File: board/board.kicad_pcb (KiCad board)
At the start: 2 copper layers, 21 x 13 mm, 1 part

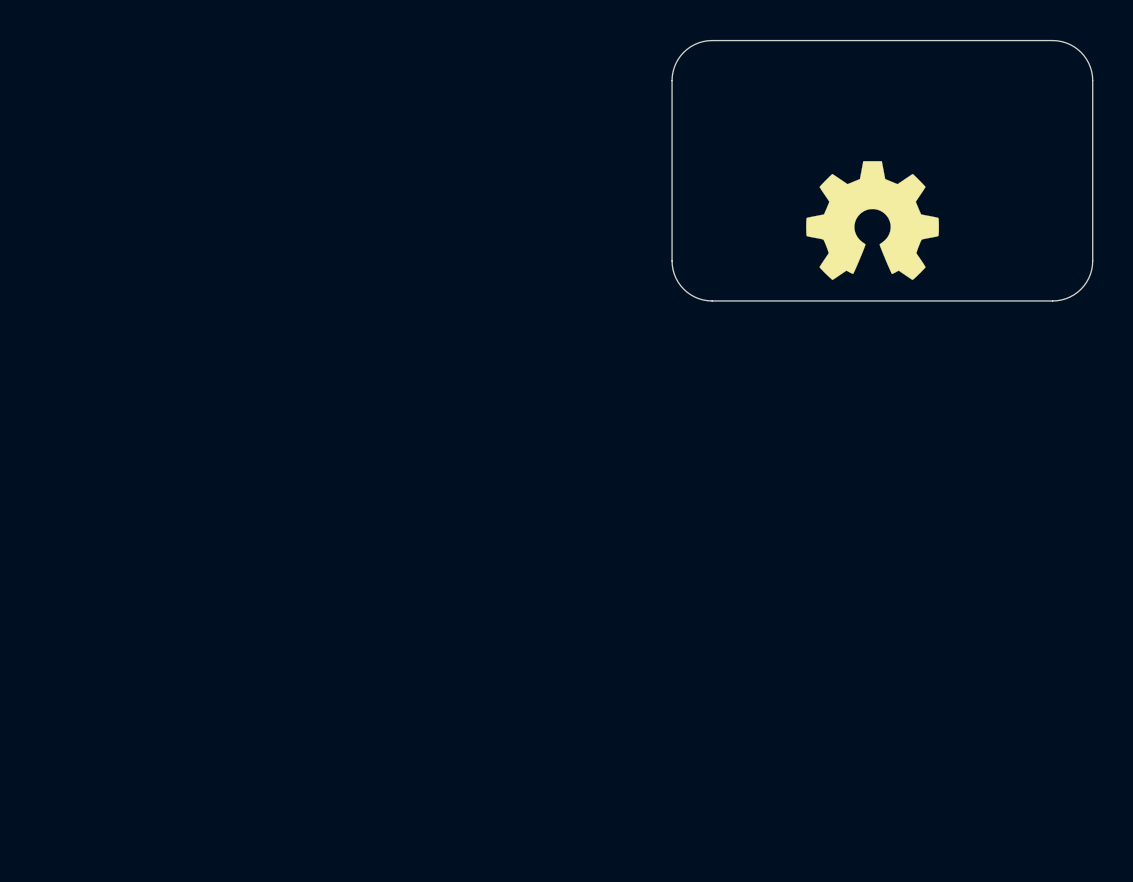
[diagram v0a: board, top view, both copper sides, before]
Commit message: imported legacy version
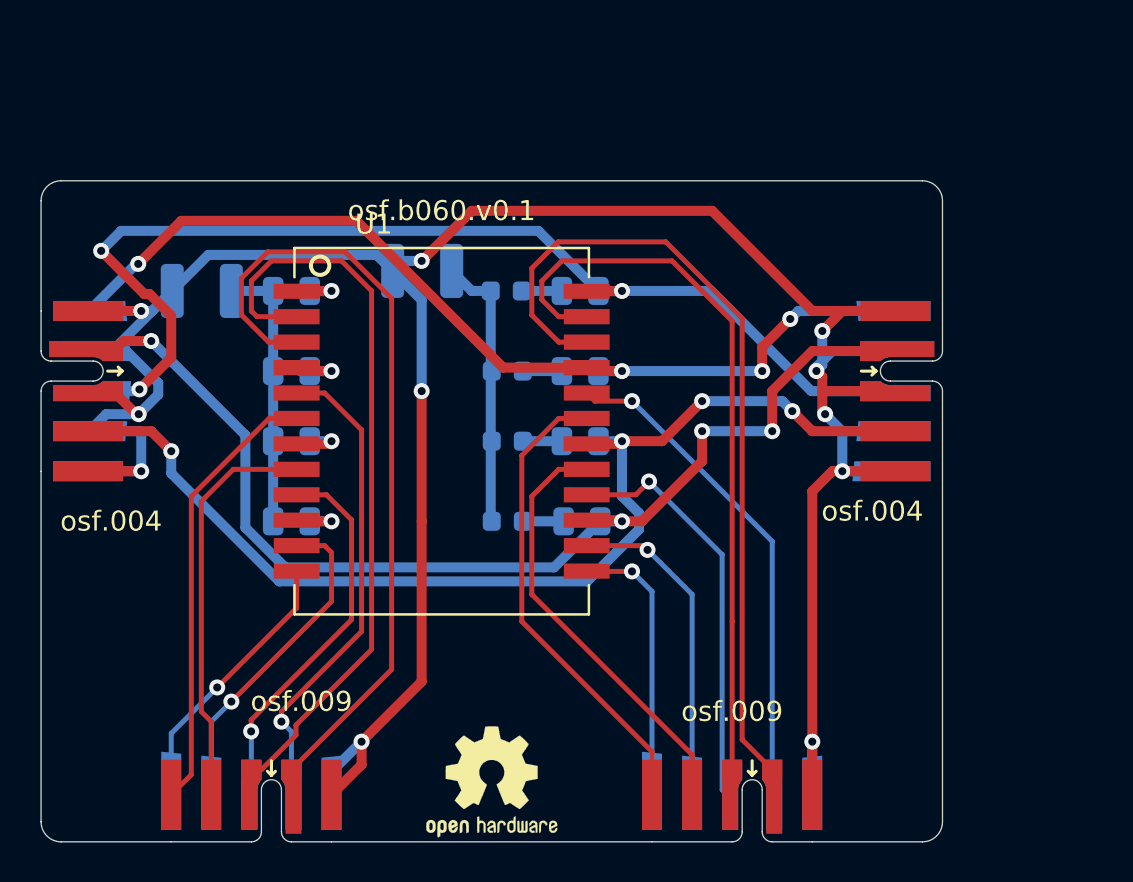
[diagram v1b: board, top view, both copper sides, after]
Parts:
- removed LOGO1: Logo_Open_Hardware_Small, Symbol:OSHW-Symbol_6.7x6mm_SilkScreen
- added C1: 1nF_2kV, Capacitor_SMD:C_1210_3225Metric, B.Cu at (127.5, 101.5)
- added C2: 10nF_100V, Capacitor_SMD:C_0603_1608Metric, B.Cu at (131.7, 102.5)
- added C3: 10nF_100V, Capacitor_SMD:C_0603_1608Metric, B.Cu at (131.8, 106.5)
- added C4: 10nF_100V, Capacitor_SMD:C_0603_1608Metric, B.Cu at (131.8, 110.0)
- added C5: 10nF_100V, Capacitor_SMD:C_0603_1608Metric, B.Cu at (131.8, 114.0)
- added C6: 1nF_2kV, Capacitor_SMD:C_1210_3225Metric, B.Cu at (116.5, 102.5)
- added J1: 004_BASE-T_CT_2x3, on_edge:on_edge_2x05_device, F.Cu at (108.5, 107.5)
- added J19: 009_1000BASE-T_2x5, on_edge:on_edge_2x05_host, F.Cu at (143.0, 130.0)
- added J20: 004_BASE-T_CT_2x3, on_edge:on_edge_2x05_host, F.Cu at (153.5, 107.5)
- added J21: 009_1000BASE-T_2x5, on_edge:on_edge_2x05_host, F.Cu at (119.0, 130.0)
- added R1: 75R, Resistor_SMD:R_0805_2012Metric, B.Cu at (135.4, 102.5)
- added R2: 75R, Resistor_SMD:R_0805_2012Metric, B.Cu at (135.4, 106.5)
- added R3: 75R, Resistor_SMD:R_0805_2012Metric, B.Cu at (135.4, 110.0)
- added R4: 75R, Resistor_SMD:R_0805_2012Metric, B.Cu at (135.5, 114.0)
- added R5: 75R, Resistor_SMD:R_0805_2012Metric, B.Cu at (121.0, 102.5)
- added R6: 75R, Resistor_SMD:R_0805_2012Metric, B.Cu at (121.0, 106.5)
- added R7: 75R, Resistor_SMD:R_0805_2012Metric, B.Cu at (121.0, 110.0)
- added R8: 75R, Resistor_SMD:R_0805_2012Metric, B.Cu at (121.0, 114.0)
- added U1: WE7490220122, AI-footprints:XFMR_7490220122, F.Cu at (128.5, 109.5)
- added l1: Logo_Open_Hardware_Large, Symbol:OSHW-Logo2_7.3x6mm_SilkScreen, F.Cu at (131.0, 127.0)
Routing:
- net Earth: track 0.00 -> 149.8 mm, vias 0 -> 11
- net /CT_78: track 0.00 -> 57.4 mm, vias 0 -> 3
- net /CT_36: track 0.00 -> 55.2 mm, vias 0 -> 4
- net /CT_12: track 0.00 -> 53.7 mm, vias 0 -> 4
- net /CT_45: track 0.00 -> 48.3 mm, vias 0 -> 4
- net Net-(J19-Pad2): track 0.00 -> 41.4 mm
- net Net-(J21-Pad2): track 0.00 -> 39.8 mm
- net Net-(J21-Pad3): track 0.00 -> 37.6 mm
- net Net-(J19-Pad3): track 0.00 -> 37.1 mm
- net Net-(J19-Pad7): track 0.00 -> 25.2 mm, vias 0 -> 1
- net Net-(J21-Pad7): track 0.00 -> 24.3 mm, vias 0 -> 1
- net Net-(J19-Pad5): track 0.00 -> 23.6 mm
- net Net-(J21-Pad5): track 0.00 -> 22.2 mm
- net Net-(J19-Pad4): track 0.00 -> 21.5 mm
- net Net-(J19-Pad8): track 0.00 -> 21.0 mm, vias 0 -> 1
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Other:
- board size 21 x 13 mm -> 45 x 33 mm
- rule pad_to_mask_clearance: 0 -> 0.051
- board text added: "osf.004"
- board text added: "osf.009"
- board text added: "osf.b060.v0.1"
